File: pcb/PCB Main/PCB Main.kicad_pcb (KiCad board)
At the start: 2 copper layers, 36 parts, among them CN1 Conn_ARM_JTAG_SWD_10, J1 Conn_01x03, J2 Conn_01x02, J3 Conn_01x02, J4 Conn_01x02, SW1 SW_Push, U1 STM32WB55RGVx, U2 AEM10941, U3 INA3221, Y1 32MHz, Y2 32.768kHz

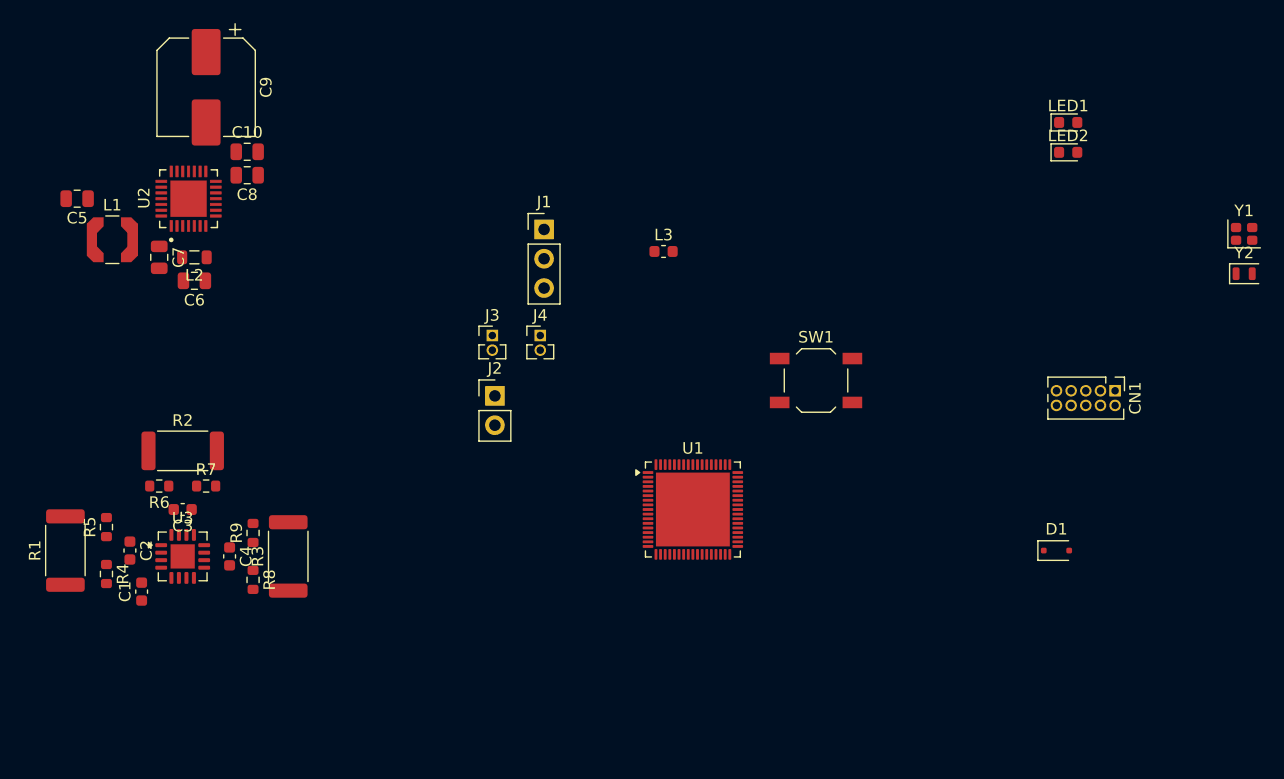
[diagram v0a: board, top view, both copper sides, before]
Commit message: PCB casi lista
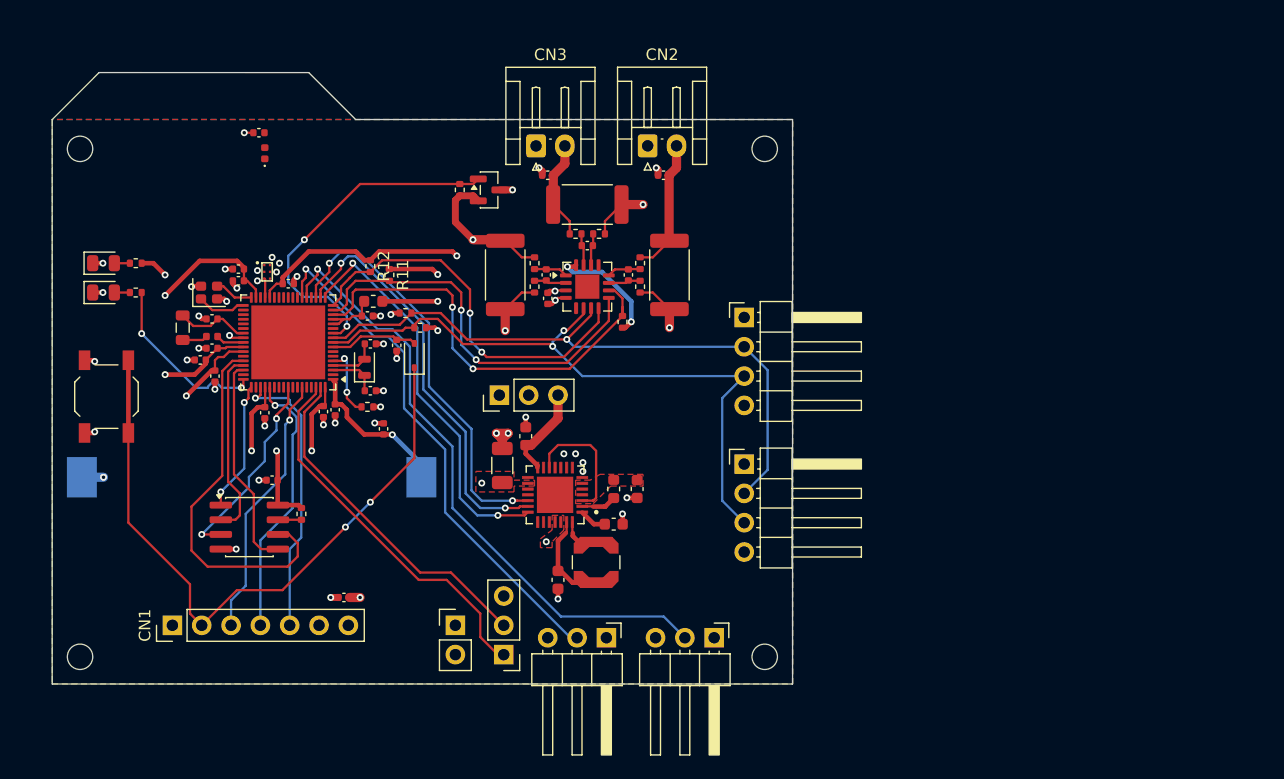
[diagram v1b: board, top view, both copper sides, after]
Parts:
- removed J2: Conn_01x02, Connector_PinHeader_2.54mm:PinHeader_1x02_P2.54mm_Vertical
- removed J3, J4: Conn_01x02, Connector_PinHeader_1.27mm:PinHeader_1x02_P1.27mm_Vertical
- added BT1: CR2032, PZG_Batteries:SMTU2032C, B.Cu at (38.5, 52.6)
- added C11: 100nF, Capacitor_SMD:C_0402_1005Metric, F.Cu at (46.5, 63.0)
- added C12: 100nF, Capacitor_SMD:C_0402_1005Metric, F.Cu at (44.7, 46.9)
- added C13: 100nF, Capacitor_SMD:C_0402_1005Metric, F.Cu at (35.3, 43.8)
- added C14: 100nF, Capacitor_SMD:C_0402_1005Metric, F.Cu at (41.7, 35.8)
- added C15: 4.7uF, Capacitor_SMD:C_0402_1005Metric, F.Cu at (34.0, 42.4)
- added C16: 100nF, Capacitor_SMD:C_0402_1005Metric, F.Cu at (35.1, 41.4)
- added C17: 100nF, Capacitor_SMD:C_0402_1005Metric, F.Cu at (48.5, 38.6)
- added C18: 100nF, Capacitor_SMD:C_0402_1005Metric, F.Cu at (39.6, 47.0)
- added C19: 100nF, Capacitor_SMD:C_0402_1005Metric, F.Cu at (37.3, 34.5)
- added C20: 100pF, Capacitor_SMD:C_0402_1005Metric, F.Cu at (37.3, 35.6)
- added C21: 100nF, Capacitor_SMD:C_0402_1005Metric, F.Cu at (45.7, 46.7)
- added C22: 4.7uF, Capacitor_SMD:C_0402_1005Metric, F.Cu at (35.1, 38.9)
- added C23: 100nF, Capacitor_SMD:C_0402_1005Metric, F.Cu at (51.1, 41.1)
- added C24: 15pF, Capacitor_SMD:C_0402_1005Metric, F.Cu at (48.8, 45.1)
- added C25: 15pF, Capacitor_SMD:C_0402_1005Metric, F.Cu at (48.8, 41.0)
- added C26: 100nF, Capacitor_SMD:C_0402_1005Metric, F.Cu at (49.9, 48.4)
- added C27: 100nF, Capacitor_SMD:C_0402_1005Metric, F.Cu at (74.2, 26.4)
- added C28: 100nF, Capacitor_SMD:C_0402_1005Metric, F.Cu at (64.1, 26.4)
- added C29: 1.2pF, Capacitor_SMD:C_0402_1005Metric, F.Cu at (39.1, 22.7)
- added CN2: Conn_01x02, Connector_JST:JST_EH_S2B-EH_1x02_P2.50mm_Horizontal, F.Cu at (72.8, 23.9)
- added CN3: Conn_01x02, Connector_JST:JST_EH_S2B-EH_1x02_P2.50mm_Horizontal, F.Cu at (63.1, 23.9)
- added CN4: Conn_01x04, Connector_PinHeader_2.54mm:PinHeader_1x04_P2.54mm_Horizontal, F.Cu at (81.2, 38.7)
- added CN5: Conn_01x04, Connector_PinHeader_2.54mm:PinHeader_1x04_P2.54mm_Horizontal, F.Cu at (81.2, 51.4)
- added CN6: Conn_01x03, Connector_PinHeader_2.54mm:PinHeader_1x03_P2.54mm_Horizontal, F.Cu at (78.6, 66.5)
- added CN7: Conn_01x03, Connector_PinHeader_2.54mm:PinHeader_1x03_P2.54mm_Horizontal, F.Cu at (69.2, 66.5)
- added CN8: Conn_01x03, Connector_PinHeader_2.54mm:PinHeader_1x03_P2.54mm_Vertical, F.Cu at (60.3, 67.9)
- added CN9: Conn_01x02, Connector_PinHeader_2.54mm:PinHeader_1x02_P2.54mm_Vertical, F.Cu at (56.1, 65.4)
- added FLT1: Low_Pass_Filter_2.4GHz_50R, MLPF-WB55-01E3:MLPF-WB55-01E3, F.Cu at (39.9, 34.8)
- added H1: MountingHole, MountingHole:MountingHole_2.2mm_M2, F.Cu at (23.6, 24.1)
- added H2: MountingHole, MountingHole:MountingHole_2.2mm_M2, F.Cu at (82.9, 24.1)
- added H3: MountingHole, MountingHole:MountingHole_2.2mm_M2, F.Cu at (82.9, 68.1)
- added H4: MountingHole, MountingHole:MountingHole_2.2mm_M2, F.Cu at (23.6, 68.1)
- added L4: 10nH, Inductor_SMD:L_0402_1005Metric, F.Cu at (35.1, 40.4)
- added L5: 10uH, Inductor_SMD:L_0805_2012Metric, F.Cu at (32.5, 39.6)
- added L6: 3.6nH, LED_SMD:LED_0402_1005Metric, F.Cu at (39.6, 24.5)
- added Q1: AO3401A, Package_TO_SOT_SMD:SOT-23, F.Cu at (59.1, 27.7)
- added R10: 10k, Resistor_SMD:R_0402_1005Metric, F.Cu at (70.6, 39.1)
- added R11: 10k, Resistor_SMD:R_0402_1005Metric, F.Cu at (50.4, 35.1)
- added R12: 10k, Resistor_SMD:R_0402_1005Metric, F.Cu at (48.8, 34.3)
- added R13: 10k, Resistor_SMD:R_0402_1005Metric, F.Cu at (48.5, 46.5)
- added R14: 10k, Resistor_SMD:R_0402_1005Metric, F.Cu at (53.1, 39.6)
- added R15: 10k, Resistor_SMD:R_0402_1005Metric, F.Cu at (51.8, 38.4)
- added R16: 470, Resistor_SMD:R_0402_1005Metric, F.Cu at (28.4, 34.0)
- added R17: 300, Resistor_SMD:R_0402_1005Metric, F.Cu at (28.4, 36.6)
- added R18: 100k, Resistor_SMD:R_0402_1005Metric, F.Cu at (56.5, 27.7)
- added R19: 10k, Resistor_SMD:R_0402_1005Metric, F.Cu at (42.8, 55.8)
- added U4: MB85RS256B, Package_SO:SOIC-8_3.9x4.9mm_P1.27mm, F.Cu at (38.3, 56.9)
- C1: value 0.1uF -> 100nF; footprint Capacitor_SMD:C_0603_1608Metric -> Capacitor_SMD:C_0402_1005Metric
- C10: value 10uF -> 100nF; footprint Capacitor_SMD:C_0805_2012Metric -> Capacitor_SMD:C_0402_1005Metric
- C2, C3, C4: value 33nF -> 100nF; footprint Capacitor_SMD:C_0603_1608Metric -> Capacitor_SMD:C_0402_1005Metric
- C5, C6, C7, C8: footprint Capacitor_SMD:C_0805_2012Metric -> Capacitor_SMD:C_0603_1608Metric
- C9: value 220uF -> 150uF; footprint Capacitor_SMD:CP_Elec_8x6.2 -> Capacitor_SMD:C_1206_3216Metric
- CN1: value Conn_ARM_JTAG_SWD_10 -> Conn_01x07; footprint Connector_PinHeader_1.27mm:PinHeader_2x05_P1.27mm_Vertical -> Connector_PinHeader_2.54mm:PinHeader_1x07_P2.54mm_Vertical
- D1: value BAT54J -> D_Schottky; footprint Diode_SMD:D_SOD-323F -> Diode_SMD:D_SOD-323
- L2: footprint Inductor_SMD:L_0805_2012Metric -> Inductor_SMD:L_0603_1608Metric
- L3: value 600 -> 600@100MHz
- LED1: value GREEN -> Green; footprint LED_SMD:LED_0603_1608Metric -> LED_SMD:LED_0805_2012Metric
- LED2: value BLUE -> White; footprint LED_SMD:LED_0603_1608Metric -> LED_SMD:LED_0805_2012Metric
- R1, R2, R3: value 0.1 -> 0.33
- R4, R5, R6, R7, R8, R9: footprint Resistor_SMD:R_0603_1608Metric -> Resistor_SMD:R_0402_1005Metric
- SW1: value SW_Push -> SW_Reset
- moved X1 89.8 mm to (34.8, 36.6)
- moved LED1 84.5 mm to (25.7, 34.0)
- moved LED2 84.4 mm to (25.7, 36.6)
- moved CN1 84.2 mm to (31.6, 65.4), turned to 90 degrees
- moved X2 76.6 mm to (48.3, 43.1), turned to 90 degrees
- moved SW1 61.5 mm to (25.9, 45.6), turned to 90 degrees
- moved D1 58.1 mm to (52.6, 42.0), turned to 90 degrees
- moved R1 57.5 mm to (74.7, 35.1), turned to -90 degrees
- moved R4 53.5 mm to (72.1, 34.0), turned to 90 degrees
- moved C5 53.2 mm to (65.0, 61.5), turned to -90 degrees
- moved R5 50.7 mm to (72.1, 36.1), turned to -90 degrees
- moved L1 50.4 mm to (68.3, 59.9), turned to -90 degrees
- moved C2 49.3 mm to (71.1, 35.1), turned to 90 degrees
- moved C7 45.7 mm to (69.8, 56.6), turned to 0 degrees
- moved C1 43.4 mm to (64.1, 37.1), turned to -90 degrees
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- renumbered Y1 to X1, Y2 to X2
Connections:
- net /Power Management/BAT+ renamed VBAT
- net /Power Management/PV+ renamed VSRC
- net /STM32WB55RG/OSC32_IN renamed /STM32WB55RG/LSE_IN
- net /STM32WB55RG/OSC32_OUT renamed /STM32WB55RG/LSE_OUT
- net /STM32WB55RG/OSC_IN renamed /STM32WB55RG/HSE_IN
- net /STM32WB55RG/OSC_OUT renamed /STM32WB55RG/HSE_OUT
- net /STM32WB55RG/SWCLK renamed SWCLK
- net S0 renamed S0_AEM
- net S1 renamed S1_AEM
- net S2 renamed S2_AEM
- C10 pad 1: /Power Management/BATT -> +3.3V
- C9 pad 1: GND -> /Power Management/BATT
- C9 pad 2: /Power Management/BATT -> GND
- CN1 pad 2: /STM32WB55RG/SWDIO -> NRST
- CN1 pad 3: GND -> SWO
- CN1 pad 5: GND -> SWDIO
- CN1 pad 6: /STM32WB55RG/SWO -> GND
- CN1 pad 7: unconnected-(CN1-KEY-Pad7) -> 3V3_EXT
- D1 pad 1: /STM32WB55RG/NRST -> NRST
- J1 pad 1: /Power Management/3V3_EXT -> 3V3_EXT
- J1 pad 2: +3.3V -> /Power Management/3V3
- L1 pad 1: Net-(U2-BUFSRC) -> Net-(U2-SWBOOST)
- L1 pad 2: Net-(U2-SWBOOST) -> Net-(U2-BUFSRC)
- LED2 pad 1: /STM32WB55RG/USER_LED -> GND
- R3 pad 1: /Power Management/HVOUT -> /Power Management/3V3
- R3 pad 2: /Power Management/3V3 -> +3.3V
- R8 pad 2: /Power Management/HVOUT -> /Power Management/3V3
- R9 pad 2: /Power Management/3V3 -> +3.3V
- SW1 pad 2: /STM32WB55RG/NRST -> NRST
- U1 pad 1: VBATT -> VBAT_BACKUP
- U1 pad 10: unconnected-(U1-PC1-Pad10) -> SDA
- U1 pad 11: unconnected-(U1-PC2-Pad11) -> GATE_SENS
- U1 pad 15: unconnected-(U1-PA0-Pad15) -> PV_INA
- U1 pad 16: unconnected-(U1-PA1-Pad16) -> CRI_INA
- U1 pad 17: /STM32WB55RG/DFR0198 -> WAR_INA
- U1 pad 22: unconnected-(U1-PA7-Pad22) -> DFR0198
- U1 pad 23: /STM32WB55RG/SEN0308 -> SEN0308
- U1 pad 47: unconnected-(U1-PB13-Pad47) -> SCK
- U1 pad 48: unconnected-(U1-PB14-Pad48) -> MISO
- U1 pad 49: unconnected-(U1-PB15-Pad49) -> MOSI
- U1 pad 51: unconnected-(U1-PA10-Pad51) -> /STM32WB55RG/USER_LED
- U1 pad 52: unconnected-(U1-PA11-Pad52) -> CS_FRAM
- U1 pad 54: /STM32WB55RG/SWDIO -> SWDIO
- U1 pad 6: SCL -> unconnected-(U1-PB8-Pad6)
- U1 pad 60: unconnected-(U1-PC12-Pad60) -> WP_FRAM
- U1 pad 63: /STM32WB55RG/SWO -> SWO
- U1 pad 65: /STM32WB55RG/USER_LED -> unconnected-(U1-PB5-Pad65)
- U1 pad 66: /STM32WB55RG/USART_RX -> USART_RX
- U1 pad 67: /STM32WB55RG/USART_TX -> USART_TX
- U1 pad 7: SDA -> unconnected-(U1-PB9-Pad7)
- U1 pad 9: unconnected-(U1-PC0-Pad9) -> SCL
- U2 pad 26: unconnected-(U2-FB_COLD-Pad26) -> /Power Management/SRC
- U3 pad 10: unconnected-(U3-PV-Pad10) -> PV_INA
- U3 pad 16: unconnected-(U3-VPU-Pad16) -> +3.3V
- U3 pad 8: unconnected-(U3-WARNING-Pad8) -> WAR_INA
- U3 pad 9: unconnected-(U3-CRITICAL-Pad9) -> CRI_INA
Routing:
- net +3.3V: track 0.00 -> 176.3 mm, vias 0 -> 16
- net VDD_SENS: track 0.00 -> 72.9 mm, vias 0 -> 1
- net /Power Management/BATT: track 0.00 -> 60.2 mm, vias 0 -> 2
- net NRST: track 0.00 -> 57.8 mm, vias 0 -> 2
- net SCL: track 0.00 -> 57.5 mm, vias 0 -> 2
- net SDA: track 0.00 -> 55.7 mm, vias 0 -> 1
- net DFR0198: track 0.00 -> 53.9 mm, vias 0 -> 1
- net SEN0308: track 0.00 -> 45.3 mm, vias 0 -> 1
- net PV_INA: track 0.00 -> 37.9 mm, vias 0 -> 2
- net S2_AEM: track 0.00 -> 36.3 mm, vias 0 -> 2
- net S1_AEM: track 0.00 -> 35.7 mm, vias 0 -> 2
- net CRI_INA: track 0.00 -> 34.8 mm, vias 0 -> 2
- net S0_AEM: track 0.00 -> 34.8 mm, vias 0 -> 2
- net WAR_INA: track 0.00 -> 33.7 mm, vias 0 -> 2
- net GND: track 0.00 -> 32.9 mm, vias 0 -> 46
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- added copper zone on F.Cu, net /Power Management/BATT
- added copper zone on F.Cu, net /Power Management/BUCK
- added copper zone on F.Cu, net /Power Management/SRC
- added copper zone on B.Cu, net GND
- added copper zone on F.Cu, net GND
- added copper zone on In1.Cu, net GND
- added copper zone on In2.Cu, net GND
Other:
- board outline added: 64.1 x 53 mm
- copper layers 2 -> 4
